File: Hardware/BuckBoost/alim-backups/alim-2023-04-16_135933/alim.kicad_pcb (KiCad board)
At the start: 2 copper layers, 29 parts, among them J1 Conn_01x02, J2 Conn_01x02, J3 Conn_01x02, J4 Conn_01x02, U1 MIC3172YM, U2 MIC3172YM

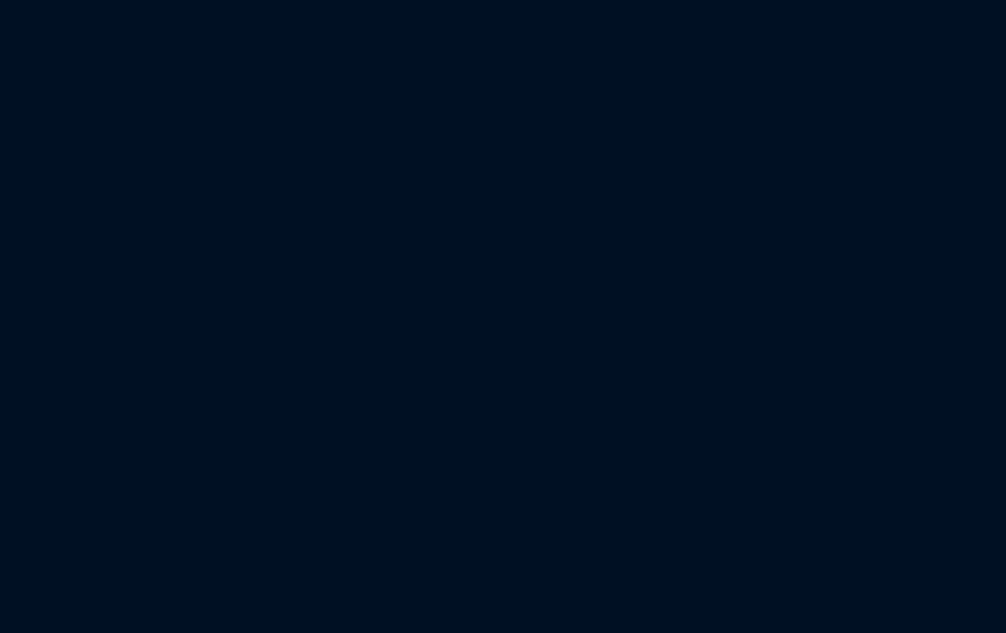
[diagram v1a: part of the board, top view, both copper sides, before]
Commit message: Update PCB
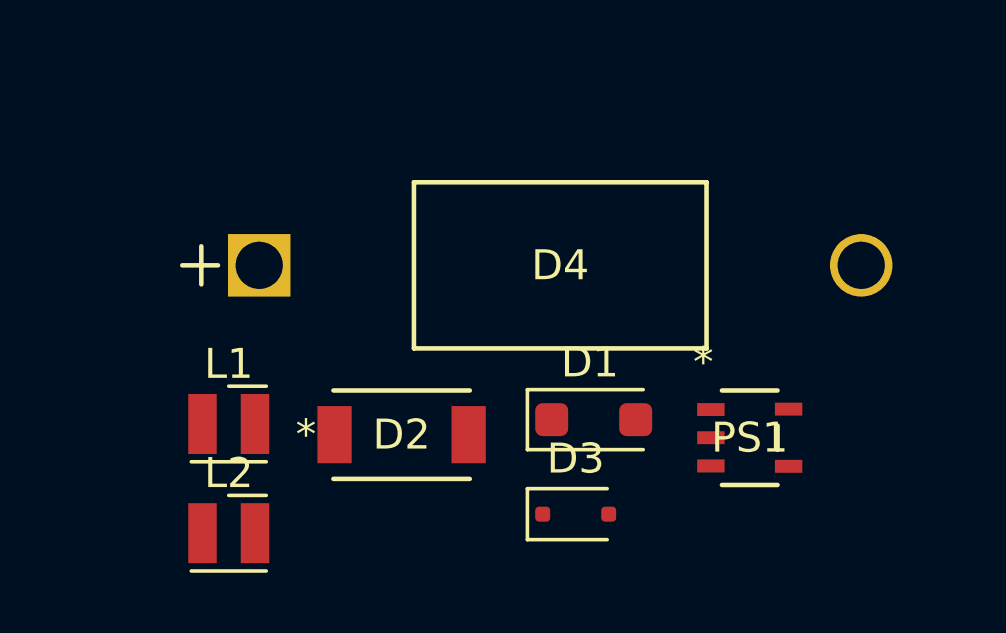
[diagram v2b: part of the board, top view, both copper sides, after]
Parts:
- added D1: 1N4148, Diode_SMD:D_SOD-123F, F.Cu at (159.2, 73.7)
- added D2: FSV330AF, Footprints_Balise:DO-214AD_ONS, F.Cu at (152.8, 74.2)
- added D3: 1N4148, Diode_SMD:D_SOD-323F, F.Cu at (158.6, 76.9)
- added D4: FSV330AF, Footprints_Balise:DIODE_1N5822-T_DIO, F.Cu at (148.1, 68.6)
- added L1: 100 µH, Inductor_SMD_Wurth:L_Wurth_WE-LQSH-2512, F.Cu at (147.1, 73.9)
- added L2: 120 µH, Inductor_SMD_Wurth:L_Wurth_WE-LQSH-2512, F.Cu at (147.1, 77.5)
- added PS1: BU33SD5WG-TR, Footprints_Balise:SSOP5_ROM, F.Cu at (164.4, 74.3)
